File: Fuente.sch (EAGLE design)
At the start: 2 parts, among them IC1 MEGA8-AI

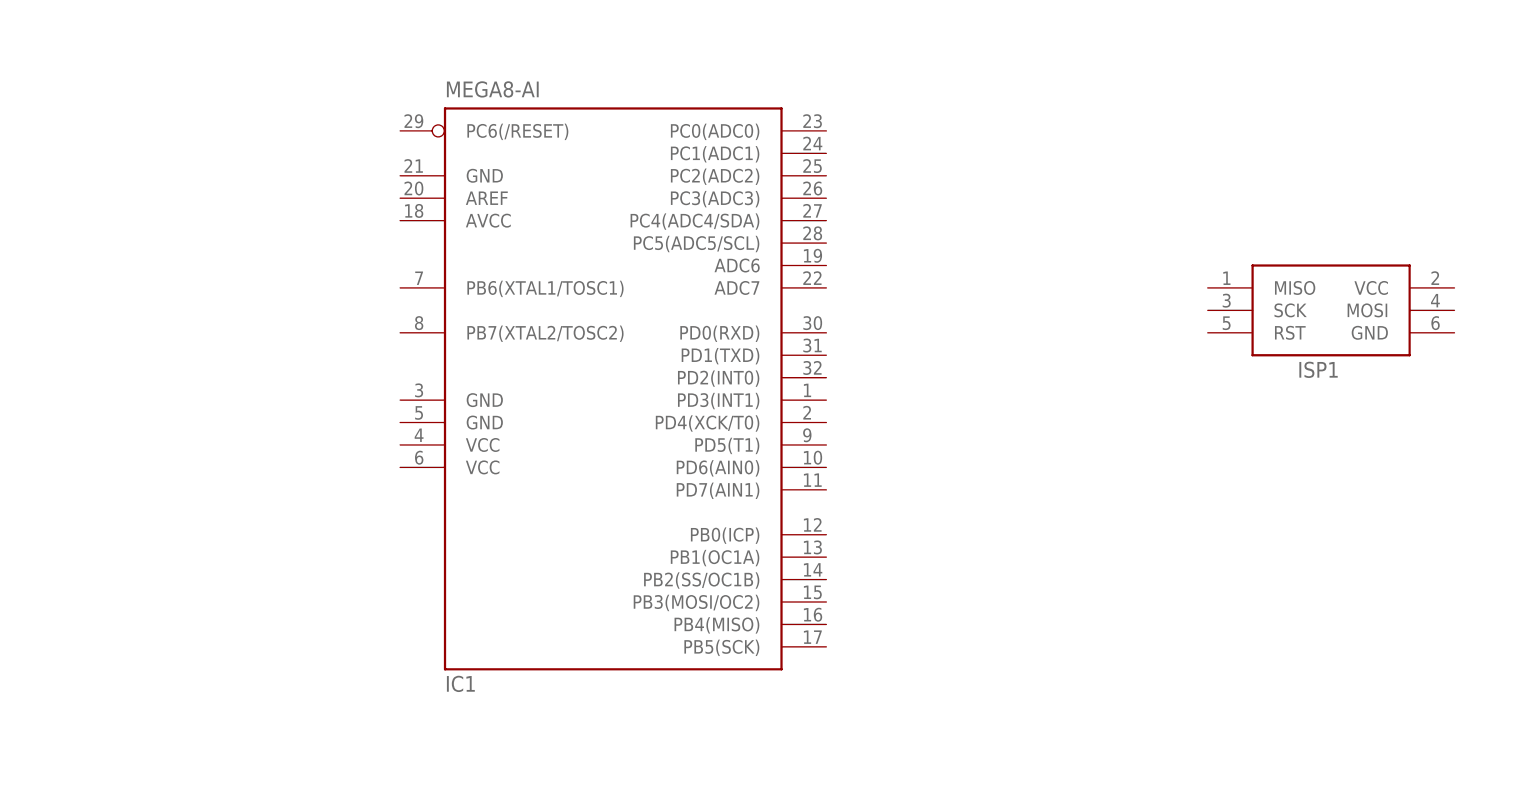
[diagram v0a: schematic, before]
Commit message: actu
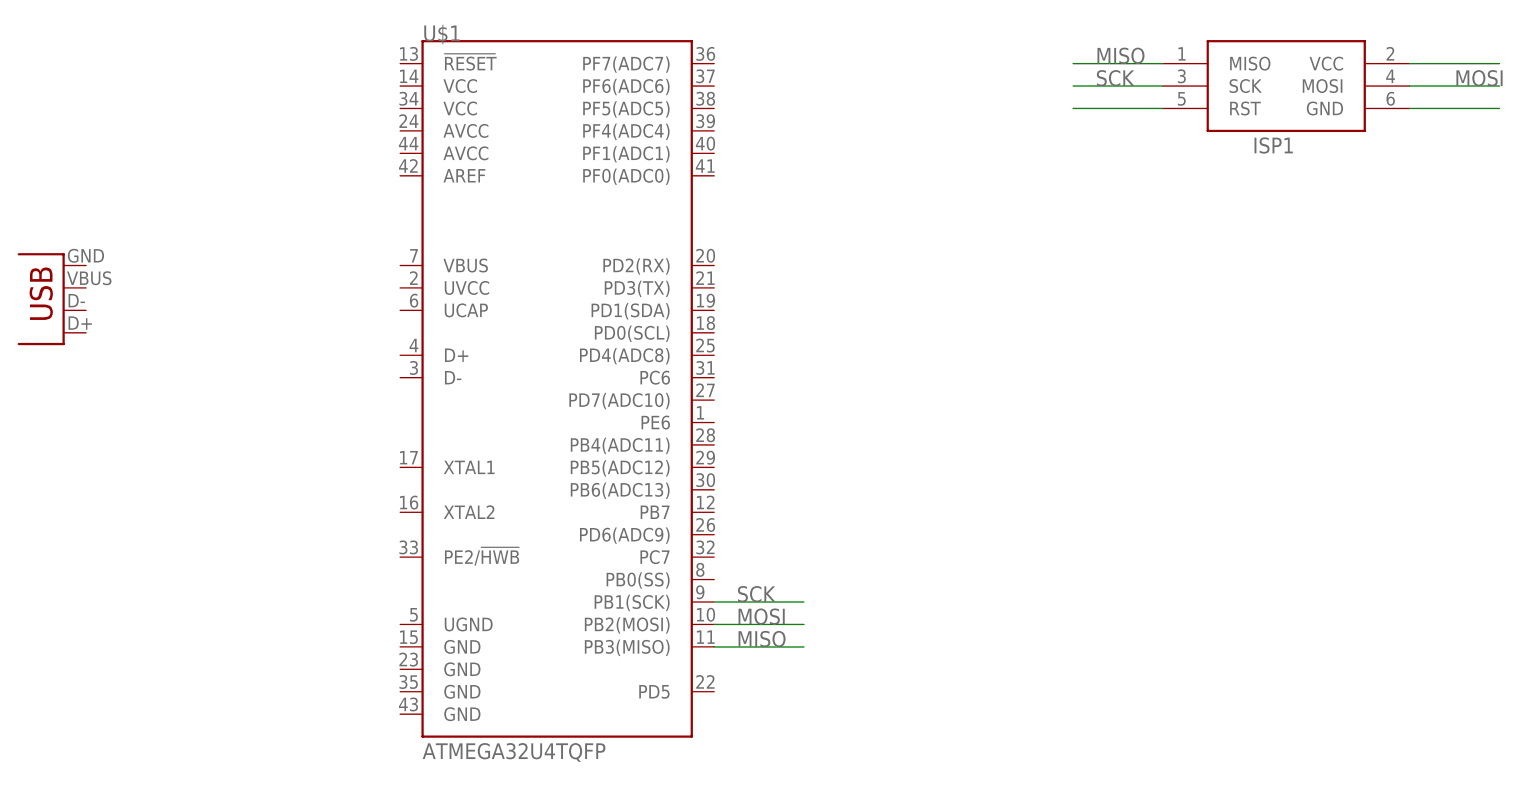
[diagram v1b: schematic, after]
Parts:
- removed IC1: MEGA8-AI, atmel:MEGA8-AI
- added JP1: USBSMD, SparkFun-Connectors:USBSMD
- added U$1: ATMEGA32U4TQFP, SparkFun-DigitalIC:ATMEGA32U4TQFP
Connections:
- new net MISO: ISP1.MISO, U$1.PB3(MISO)
- new net MOSI: ISP1.MOSI, U$1.PB2(MOSI)
- new net N$3: ISP1.RST
- new net N$4: ISP1.VCC
- new net N$6: ISP1.GND
- new net SCK: ISP1.SCK, U$1.PB1(SCK)
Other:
- moved on the sheet: ISP1
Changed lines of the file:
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@@
 <?xml version="1.0" encoding="utf-8"?>
 <!DOCTYPE eagle SYSTEM "eagle.dtd">
-<eagle version="6.2">
+<eagle version="6.3">
 <drawing>
 <settings>
@@
 </classes>
 <parts>
-<part name="IC1" library="atmel" deviceset="MEGA8" device="-AI"/>
 <part name="ISP1" library="adafruit" deviceset="AVRISP" device="-6"/>
+<part name="U$1" library="SparkFun-DigitalIC" deviceset="ATMEGA32U4" device="TQFP"/>
+<part name="JP1" library="SparkFun-Connectors" deviceset="USB" device="SMD"/>
 </parts>
 <sheets>
@@
 </plain>
 <instances>
-<instance part="IC1" gate="G$1" x="22.86" y="60.96"/>
-<instance part="ISP1" gate="G$1" x="104.14" y="66.04"/>
+<instance part="ISP1" gate="G$1" x="99.06" y="91.44"/>
+<instance part="U$1" gate="G$1" x="17.78" y="58.42"/>
+<instance part="JP1" gate="G$1" x="-38.1" y="71.12" rot="R180"/>
 </instances>
 <busses>
 </busses>
 <nets>
+<net name="MISO" class="0">
+<segment>
+<pinref part="ISP1" gate="G$1" pin="MISO"/>
+<wire x1="86.36" y1="93.98" x2="76.2" y2="93.98" width="0.1524" layer="91"/>
+<label x="78.74" y="93.98" size="1.778" layer="95"/>
+</segment>
+<segment>
+<pinref part="U$1" gate="G$1" pin="PB3(MISO)"/>
+<wire x1="35.56" y1="27.94" x2="45.72" y2="27.94" width="0.1524" layer="91"/>
+<label x="38.1" y="27.94" size="1.778" layer="95"/>
+</segment>
+</net>
+<net name="SCK" class="0">
+<segment>
+<pinref part="ISP1" gate="G$1" pin="SCK"/>
+<wire x1="86.36" y1="91.44" x2="76.2" y2="91.44" width="0.1524" layer="91"/>
+<label x="78.74" y="91.44" size="1.778" layer="95"/>
+</segment>
+<segment>
+<pinref part="U$1" gate="G$1" pin="PB1(SCK)"/>
+<wire x1="35.56" y1="33.02" x2="45.72" y2="33.02" width="0.1524" layer="91"/>
+<label x="38.1" y="33.02" size="1.778" layer="95"/>
+</segment>
+</net>
+<net name="N$3" class="0">
+<segment>
+<pinref part="ISP1" gate="G$1" pin="RST"/>
+<wire x1="86.36" y1="88.9" x2="76.2" y2="88.9" width="0.1524" layer="91"/>
+</segment>
+</net>
+<net name="N$4" class="0">
+<segment>
+<pinref part="ISP1" gate="G$1" pin="VCC"/>
+<wire x1="114.3" y1="93.98" x2="124.46" y2="93.98" width="0.1524" layer="91"/>
+</segment>
+</net>
+<net name="MOSI" class="0">
+<segment>
+<pinref part="ISP1" gate="G$1" pin="MOSI"/>
+<wire x1="114.3" y1="91.44" x2="124.46" y2="91.44" width="0.1524" layer="91"/>
+<label x="119.38" y="91.44" size="1.778" layer="95"/>
+</segment>
+<segment>
+<pinref part="U$1" gate="G$1" pin="PB2(MOSI)"/>
+<wire x1="35.56" y1="30.48" x2="45.72" y2="30.48" width="0.1524" layer="91"/>
+<label x="38.1" y="30.48" size="1.778" layer="95"/>
+</segment>
+</net>
+<net name="N$6" class="0">
+<segment>
+<pinref part="ISP1" gate="G$1" pin="GND"/>
+<wire x1="114.3" y1="88.9" x2="124.46" y2="88.9" width="0.1524" layer="91"/>
+</segment>
+</net>
 </nets>
 </sheet>

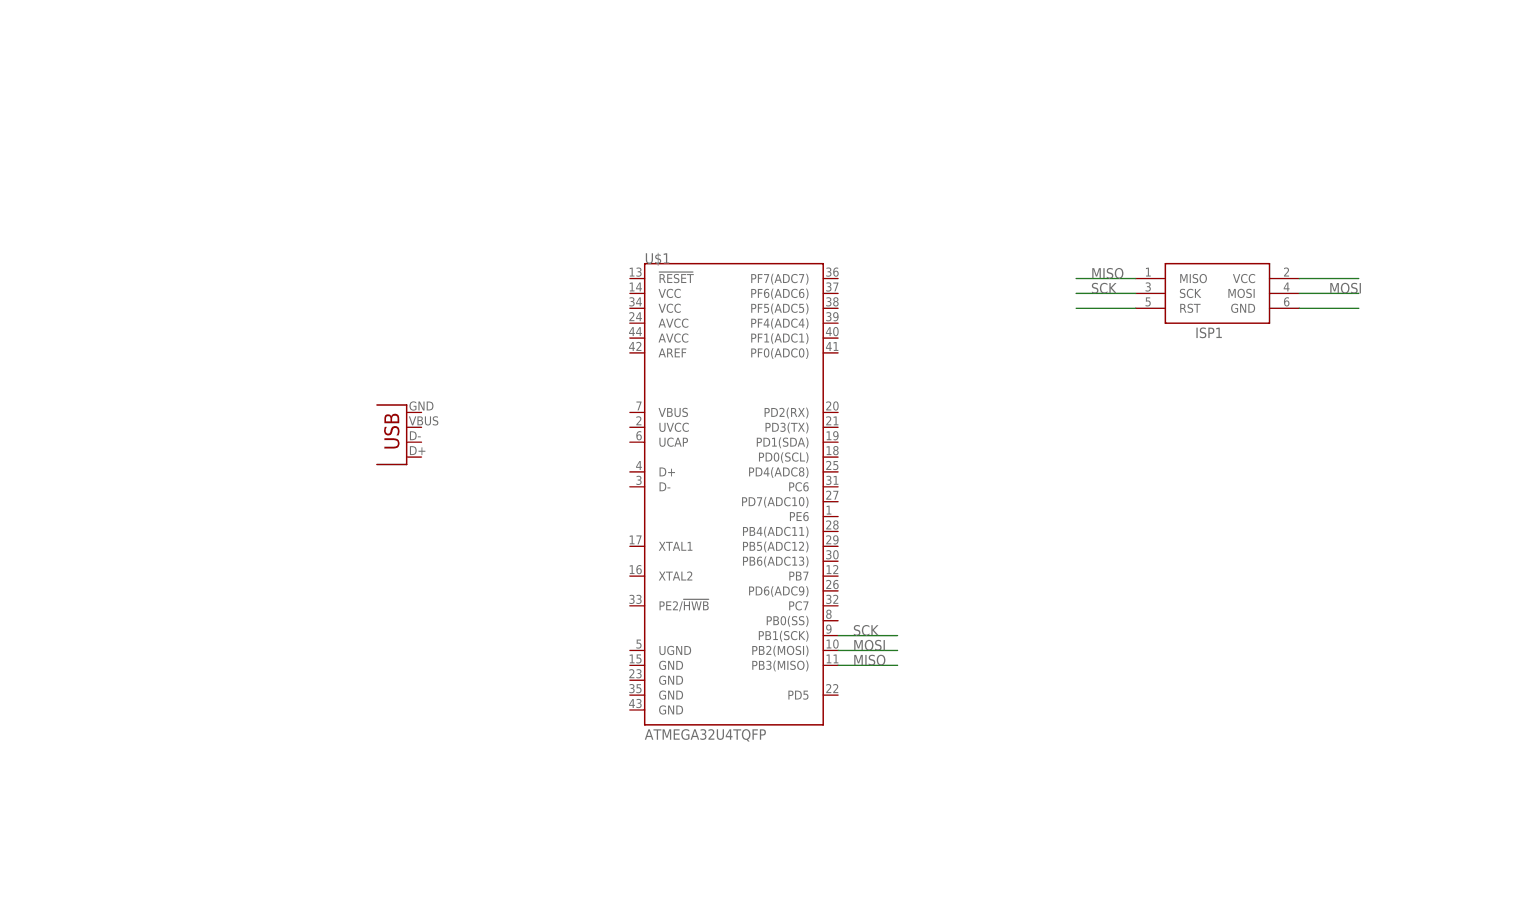
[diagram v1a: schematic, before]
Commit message: Sch updated
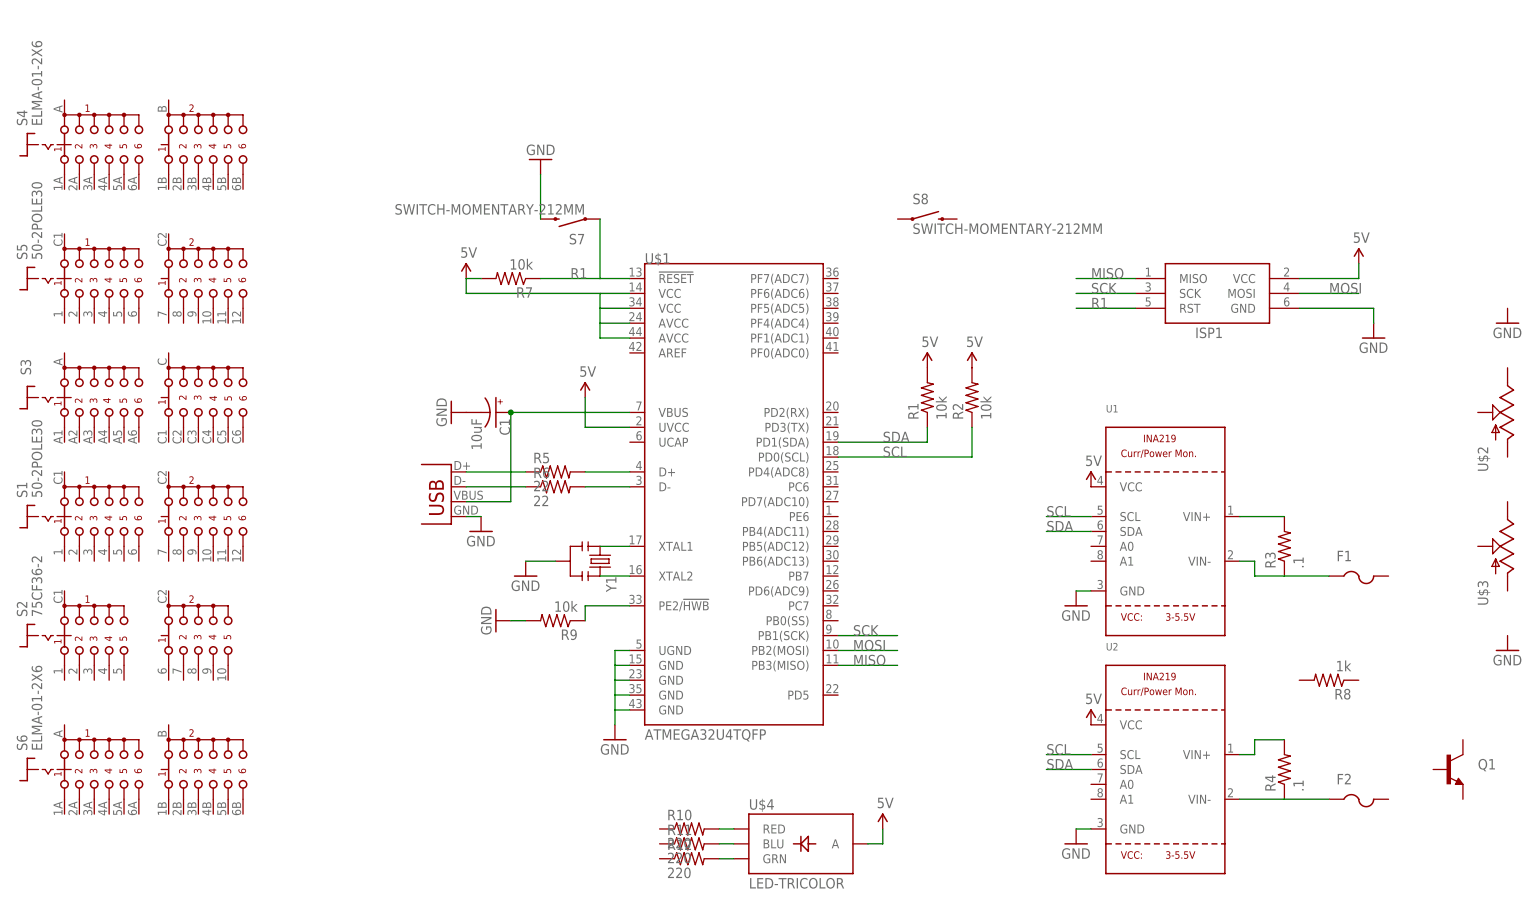
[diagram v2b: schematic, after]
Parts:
- added C1: 10uF, SparkFun-Capacitors:CAP_POLPTH2
- added F1, F2: (no value), adafruit:PTCFUSE-1812
- added Q1: (no value), SparkFun-DiscreteSemi:TRANSISTOR_NPNSOT23
- added R1, R2, R7, R9: 10k, adafruit:R-US_M0805
- added R10, R11, R12: 220, SparkFun-Resistors:RESISTOR0805-RES
- added R3, R4: .1, adafruit:R-US_R2512
- added R5, R6: 22, adafruit:R-US_0309/12
- added R8: 1k, adafruit:R-US_M0805
- added S1, S5: 50-2POLE30, switch:50-2POLE30
- added S2: 75CF36-2, switch:75CF36-2
- added S3: (no value), switch:CK102X06
- added S4, S6: ELMA-01-2X6, switch:ELMA-01-2X6
- added S7, S8: SWITCH-MOMENTARY-212MM, SparkFun-Electromechanical:SWITCH-MOMENTARY-212MM
- added U$2, U$3: (no value), SparkFun-Electromechanical:POT-RV16AF-20
- added U$4: LED-TRICOLOR, SparkFun-LED:LED-TRICOLOR
- added U1, U2: (no value), microbuilder:INA219
- added Y1: (no value), SparkFun-FreqCtrl:RESONATORPTH
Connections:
- new net 5V: ISP1.VCC, R1.2, R2.2, R7.2, U$1.AVCC@24, U$1.AVCC@44, U$1.UVCC, U$1.VCC@14, U$1.VCC@34, U$4.A, U1.VCC, U2.VCC
- new net GND: C1.-, ISP1.GND, JP1.GND, R9.2, S7.2, U$1.GND@15, U$1.GND@23, U$1.GND@35, U$1.GND@43, U$1.UGND, U1.GND, U2.GND, Y1.2
- new net N$1: R4.2, U2.VIN+
- new net N$10: R6.2, U$1.D-
- new net N$11: JP1.D-, R6.1
- new net N$12: U$1.XTAL1, Y1.1
- new net N$13: U$1.XTAL2, Y1.3
- new net N$14: R11.2, U$4.BLU
- new net N$15: R12.2, U$4.GRN
- new net N$2: F2.1, R4.1, U2.VIN-
- new net N$5: R3.2, U1.VIN+
- new net N$7: F1.1, R3.1, U1.VIN-
- new net N$8: JP1.D+, R5.1
- new net N$9: R5.2, U$1.D+
- new net R1: ISP1.RST, R7.1, S7.1, U$1.!RESET
- new net SCL: R2.1, U$1.PD0(SCL), U1.SCL, U2.SCL
- new net SDA: R1.1, U$1.PD1(SDA), U1.SDA, U2.SDA
- net N$3: now also C1.+, JP1.VBUS, U$1.VBUS; no longer ISP1.RST
- net N$4: now also R9.1, U$1.PE2/!HWB; no longer ISP1.VCC
- net N$6: now also R10.2, U$4.RED; no longer ISP1.GND
